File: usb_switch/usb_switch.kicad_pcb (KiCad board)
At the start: 4 copper layers, 50 x 50 mm, 79 parts, among them J1 Jack-DC, J2 USB_B_Micro, J3 Conn_01x04, J4 USB_A, J5 USB_A, J6 USB_A, J7 USB_A, J8 UART, U1 AMS1117-3.3, U2 USB2514B_Bi, U3 MIC2026-1BM, U4 MIC2026-1BM, U5 MCP2221-I_SL, Y1 24MHz

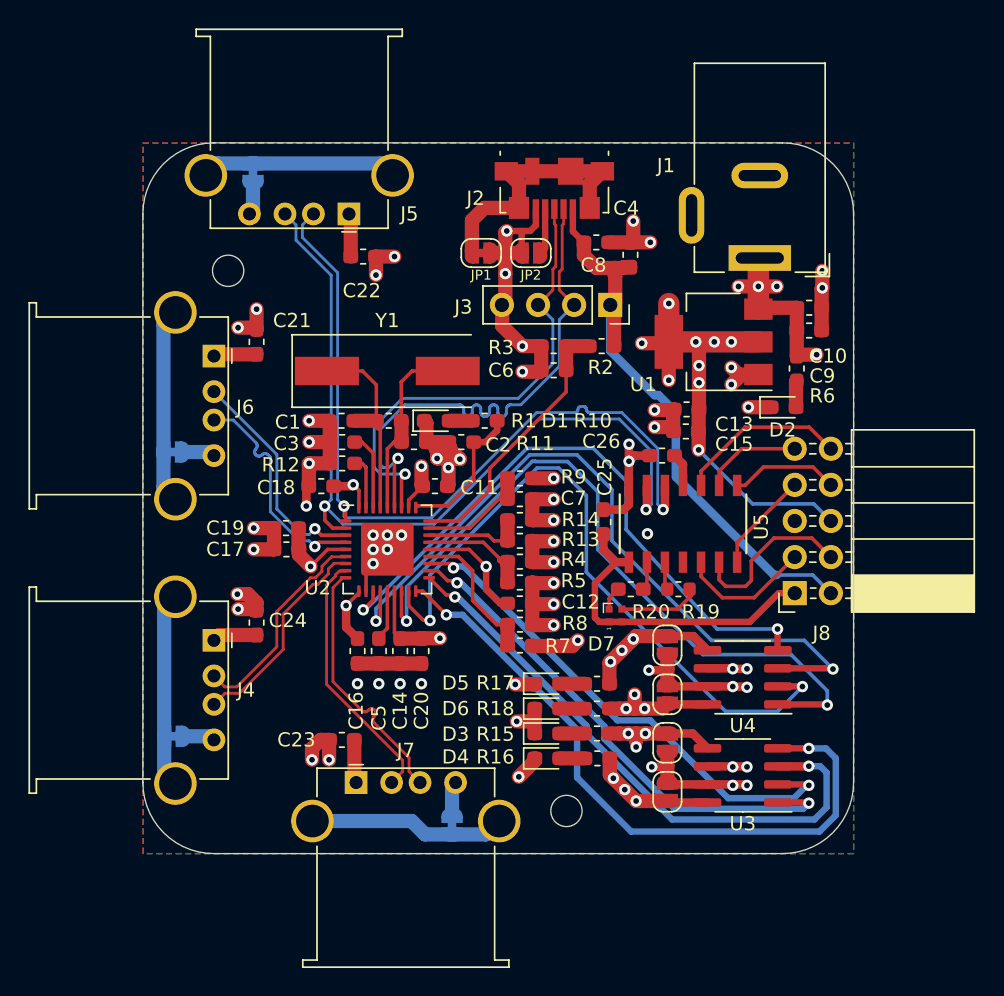
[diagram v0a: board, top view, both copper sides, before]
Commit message: ADC basics
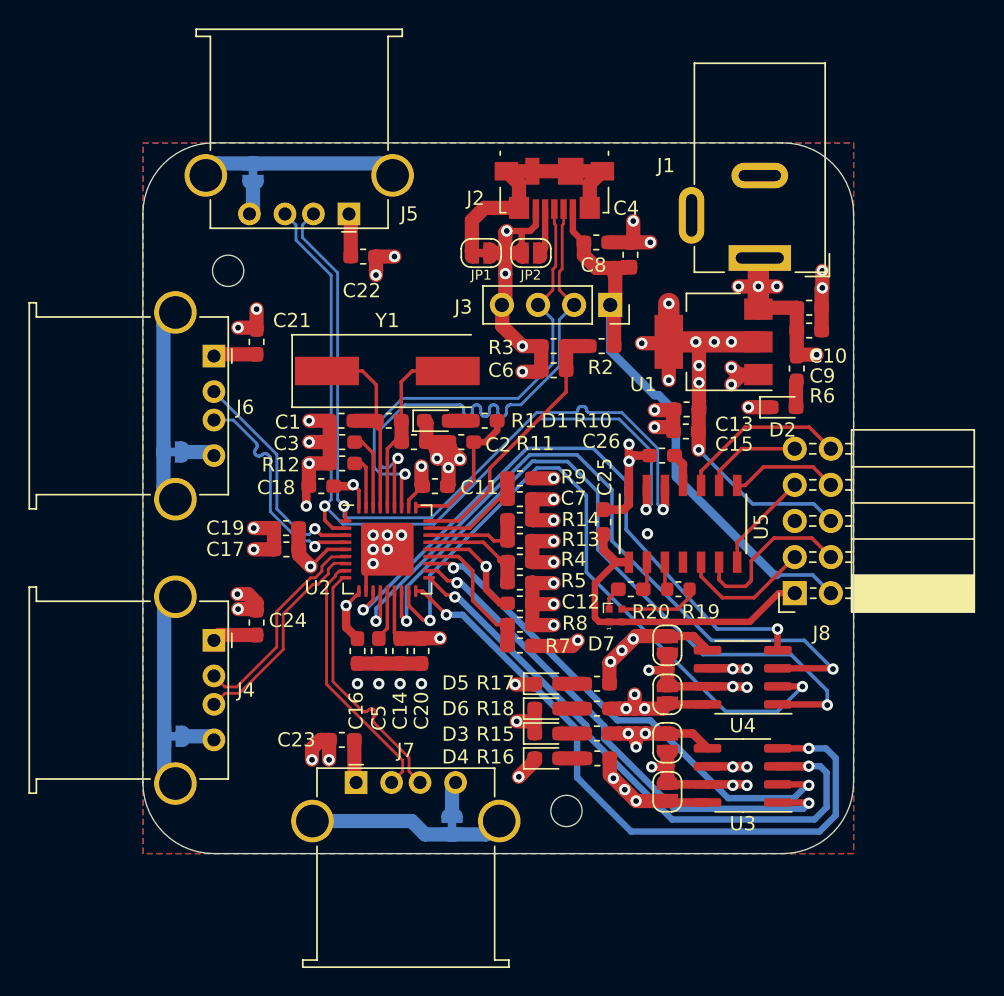
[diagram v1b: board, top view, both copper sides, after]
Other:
- net class Default removed
- net class Diff removed
- net class Power removed
